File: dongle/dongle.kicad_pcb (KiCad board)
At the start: 6 copper layers, 18 x 12 mm, 50 parts, among them SW1 GT-TC194A-H0055-L1, U1 NRF52833-QDAA-R7, U2 CH32V305GBU6, U3 SY80004DQD, X1 XL7EL89CKI-111YLC-32M, X2 XL2OI-111-8M

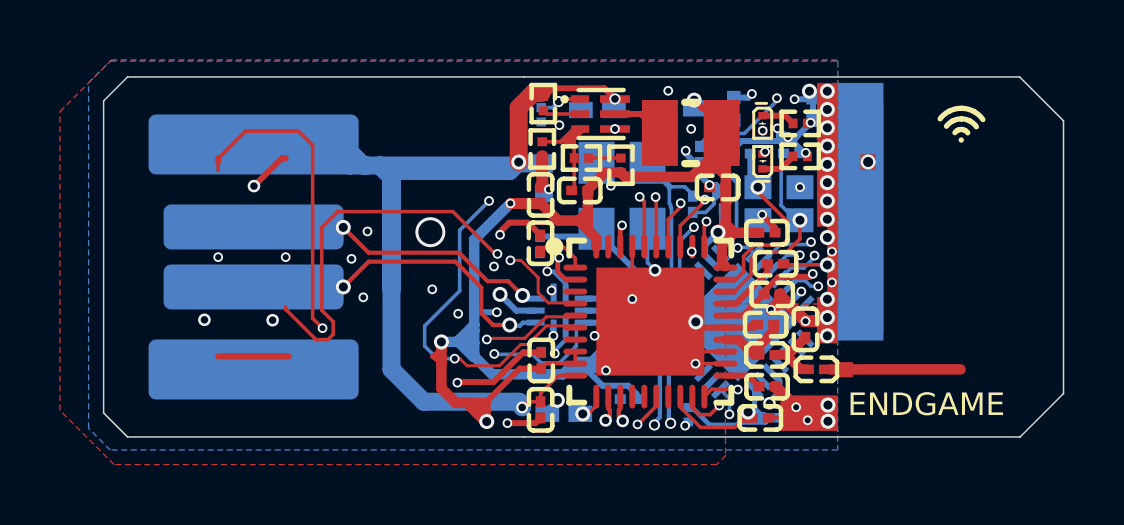
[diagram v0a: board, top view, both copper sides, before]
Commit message: feat: 1k dongle, rev5 hw (wip)
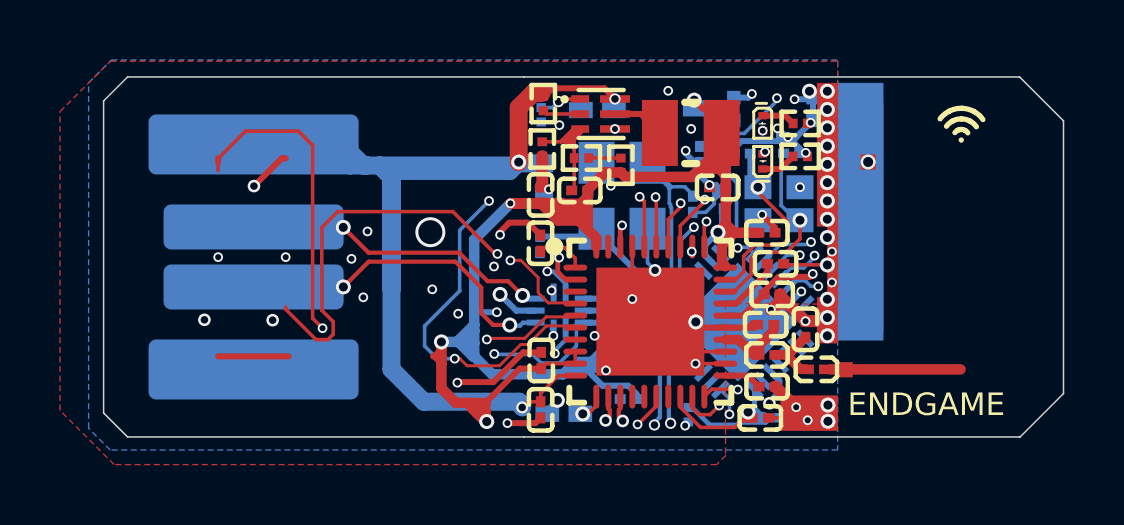
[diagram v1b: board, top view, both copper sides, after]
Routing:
- net 3V3: track 85.1 -> 88.3 mm
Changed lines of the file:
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@@
+	)
+	(segment
+		(start 191.326933 84.635989)
+		(end 191.584426 84.893481)
+		(width 0.35)
+		(layer "F.Cu")
+		(net 6)
 	)
 	(segment
@@
 	)
 	(segment
+		(start 192.342662 84.635989)
+		(end 192.575601 84.40305)
+		(width 0.35)
+		(layer "F.Cu")
+		(net 6)
+	)
+	(segment
 		(start 189.23 90.994468)
 		(end 189.034478 90.994468)
@@
 	)
 	(segment
+		(start 192.575601 84.094432)
+		(end 192.575601 83.889291)
+		(width 0.35)
+		(layer "F.Cu")
+		(net 6)
+	)
+	(segment
 		(start 187.452 89.4207)
 		(end 187.6933 89.1794)
@@
 	)
 	(segment
+		(start 191.737462 84.336632)
+		(end 192.333401 84.336632)
+		(width 0.35)
+		(layer "F.Cu")
+		(net 6)
+	)
+	(segment
 		(start 197.171625 83.386536)
 		(end 197.171625 83.161438)
@@
 	)
 	(segment
+		(start 192.333401 84.336632)
+		(end 192.575601 84.094432)
+		(width 0.35)
+		(layer "F.Cu")
+		(net 6)
+	)
+	(segment
 		(start 193.144793 83.289238)
 		(end 193.675411 83.289238)
@@
 	(segment
 		(start 191.012927 84.321982)
-		(end 191.584426 84.893481)
+		(end 191.326933 84.635989)
 		(width 0.35)
 		(layer "F.Cu")
@@
 	)
 	(segment
+		(start 191.326933 84.635989)
+		(end 192.342662 84.635989)
+		(width 0.35)
+		(layer "F.Cu")
+		(net 6)
+	)
+	(segment
 		(start 190.304904 89.8271)
 		(end 191.0207 89.8271)
@@
 	)
 	(segment
+		(start 190.999234 84.308289)
+		(end 191.709119 84.308289)
+		(width 0.35)
+		(layer "F.Cu")
+		(net 6)
+	)
+	(segment
 		(start 182.600302 89.4207)
 		(end 183.576159 89.4207)
@@
 		(start 196.453801 83.161438)
 		(end 196.387194 83.094831)
+		(width 0.35)
+		(layer "F.Cu")
+		(net 6)
+	)
+	(segment
+		(start 191.709119 84.308289)
+		(end 191.737462 84.336632)
 		(width 0.35)
 		(layer "F.Cu")
@@
 	)
 	(segment
+		(start 196.572942 82.421036)
+		(end 197.439254 81.554724)
+		(width 0.2)
+		(layer "B.Cu")
+		(net 23)
+	)
+	(segment
 		(start 197.439254 80.794724)
 		(end 197.921689 80.794724)
@@
 	(segment
 		(start 196.308073 82.421036)
-		(end 196.308073 82.407411)
+		(end 196.572942 82.421036)
 		(width 0.2)
 		(layer "B.Cu")
@@
 		(width 0.2)
 		(layer "B.Cu")
-		(net 23)
-	)
-	(segment
-		(start 196.308073 82.407411)
-		(end 197.16076 81.554724)
-		(width 0.2)
-		(layer "B.Cu")
-		(net 23)
-	)
-	(segment
-		(start 197.16076 81.554724)
-		(end 197.439254 81.554724)
-		(width 0.2)
-		(layer "B.Cu")
